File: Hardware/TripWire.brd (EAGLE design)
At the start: 37.2 x 50.3 mm, 67 parts, among them P1 LSP11, P2 LSP11, P3 LSP11, P4 LSP11, P5 LSP11, P6 LSP11, P7 LSP11, X1 GADGETEER-SOCKET

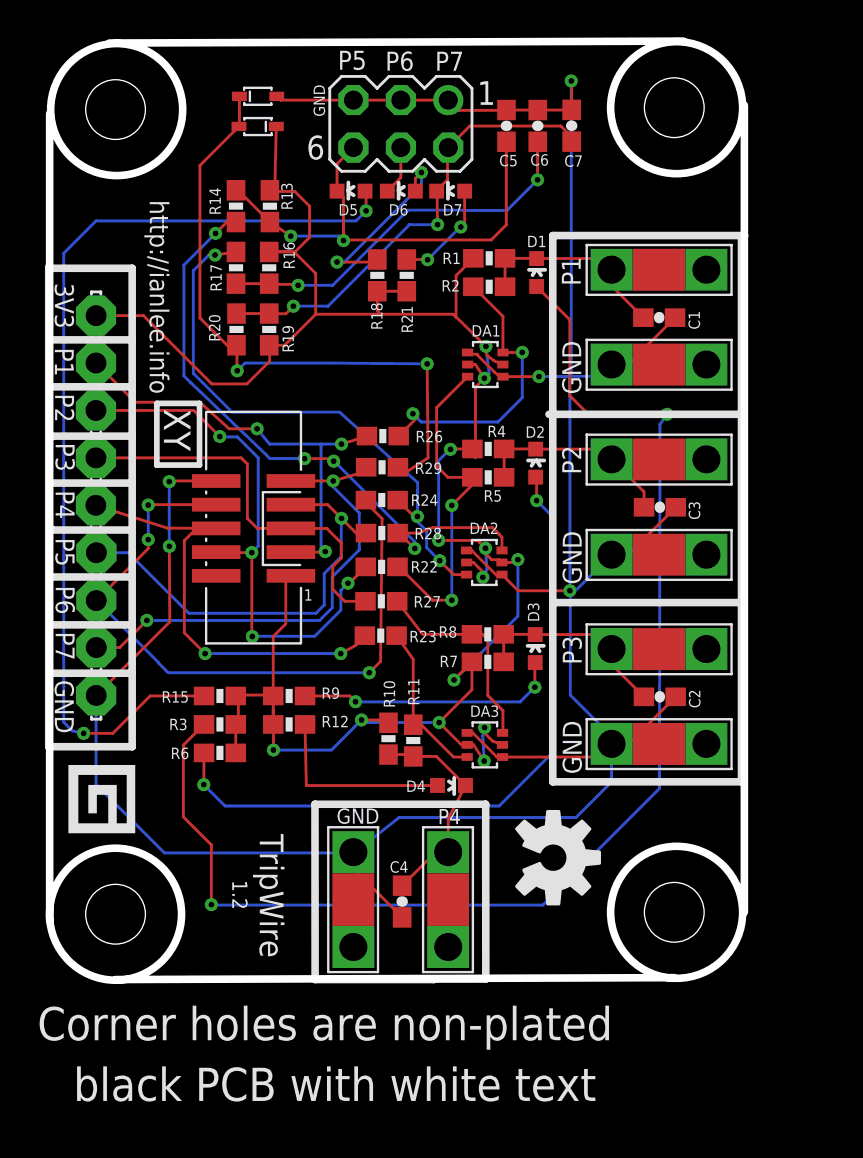
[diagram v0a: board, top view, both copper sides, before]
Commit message: Moved OSHW logo.
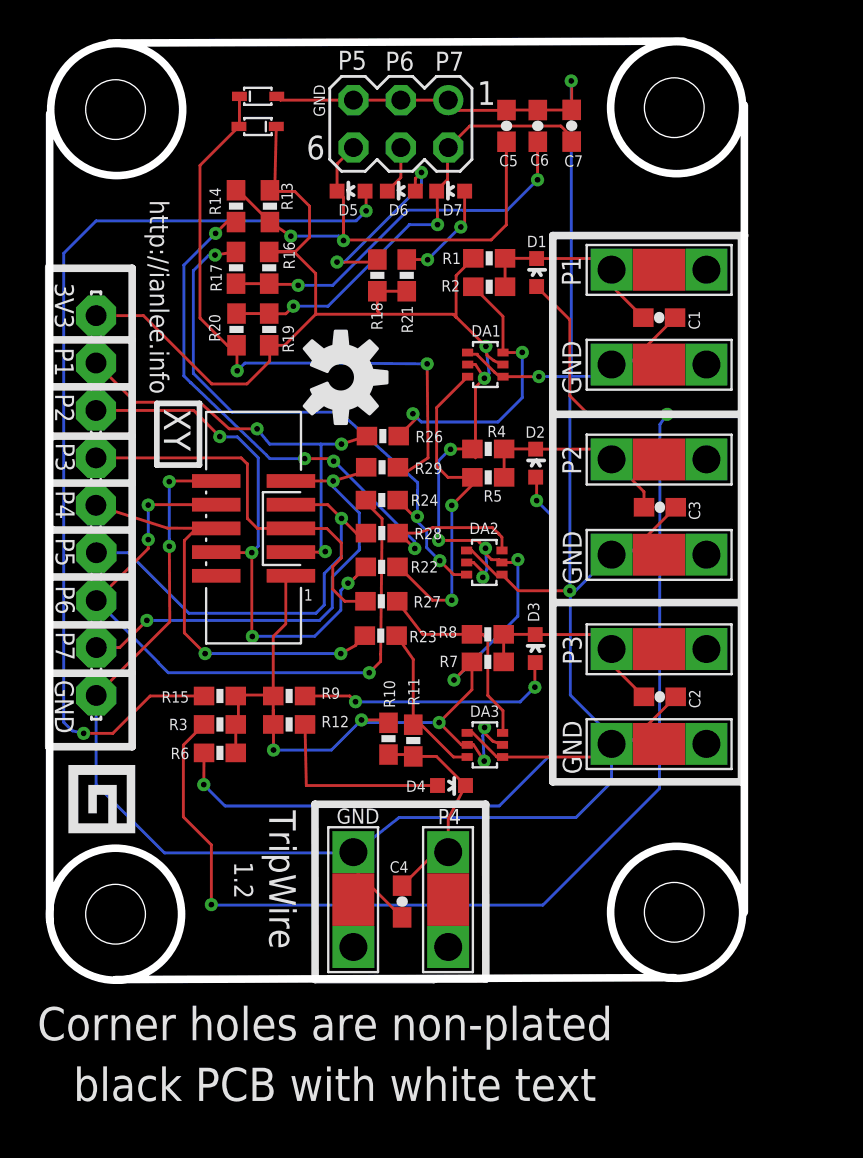
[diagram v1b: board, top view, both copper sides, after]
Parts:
- moved LOGO1 28.1 mm to (15.6, 32.3)
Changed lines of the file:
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@@
 <layer number="151" name="HeatSink" color="14" fill="1" visible="no" active="no"/>
 <layer number="199" name="Contour" color="7" fill="1" visible="no" active="no"/>
-<layer number="200" name="200bmp" color="7" fill="10" visible="yes" active="yes"/>
-<layer number="201" name="201bmp" color="15" fill="10" visible="yes" active="yes"/>
+<layer number="200" name="200bmp" color="7" fill="10" visible="no" active="yes"/>
+<layer number="201" name="201bmp" color="15" fill="10" visible="no" active="yes"/>
 <layer number="202" name="202bmp" color="7" fill="1" visible="no" active="yes"/>
 <layer number="203" name="203bmp" color="7" fill="1" visible="no" active="yes"/>
@@
 <circle x="33.6346" y="3.6016" radius="3.5355" width="0.4064" layer="20"/>
 <circle x="3.58" y="3.5" radius="3.5355" width="0.4064" layer="20"/>
-<text x="11.30401875" y="7.79131875" size="1.27" layer="21" ratio="12" rot="SR270">TripWire</text>
-<text x="9.830821875" y="5.330059375" size="0.8128" layer="21" ratio="12" rot="SR270">1.2</text>
+<text x="11.81201875" y="9.06131875" size="1.4224" layer="21" ratio="12" rot="SR270">TripWire</text>
+<text x="9.932421875" y="6.320659375" size="1.016" layer="21" ratio="12" rot="SR270">1.2</text>
 <text x="5.4102" y="41.7576" size="1.016" layer="21" ratio="12" rot="SR270">http://ianlee.info</text>
 <text x="-0.6096" y="-3.2512" size="1.778" layer="21">Corner holes are non-plated</text>
@@
 <wire x1="27.0002" y1="10.5918" x2="37.1094" y2="10.5918" width="0.4064" layer="21"/>
 <wire x1="37.1094" y1="10.5918" x2="37.1094" y2="39.8526" width="0.4064" layer="21"/>
-<wire x1="37.1856" y1="30.2768" x2="26.797" y2="30.2768" width="0.4064" layer="21"/>
+<wire x1="37.0586" y1="30.2768" x2="27.051" y2="30.2768" width="0.4064" layer="21"/>
 <wire x1="37.1856" y1="20.193" x2="27.1526" y2="20.193" width="0.4064" layer="21"/>
 <wire x1="20.6756" y1="0.0254" x2="23.41371875" y2="0.0254" width="0.4064" layer="21"/>
@@
 <attribute name="VALUE" x="2.295" y="17.7838" size="0.0254" layer="27" rot="R90"/>
 </element>
-<element name="LOGO1" library="SparkFun-Aesthetics" package="OSHW-LOGO-M" value="OSHW-LOGOM" x="27.0256" y="6.5278" rot="R270"/>
+<element name="LOGO1" library="SparkFun-Aesthetics" package="OSHW-LOGO-M" value="OSHW-LOGOM" x="15.6464" y="32.258" rot="R270"/>
 <element name="R22" library="SparkFun-Resistors" package="0603-RES" value="10" x="17.833340625" y="22.10561875" smashed="yes">
 <attribute name="NAME" x="19.382740625" y="21.80081875" size="0.6096" layer="25" font="vector"/>
